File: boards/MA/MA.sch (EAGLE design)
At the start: 14 parts

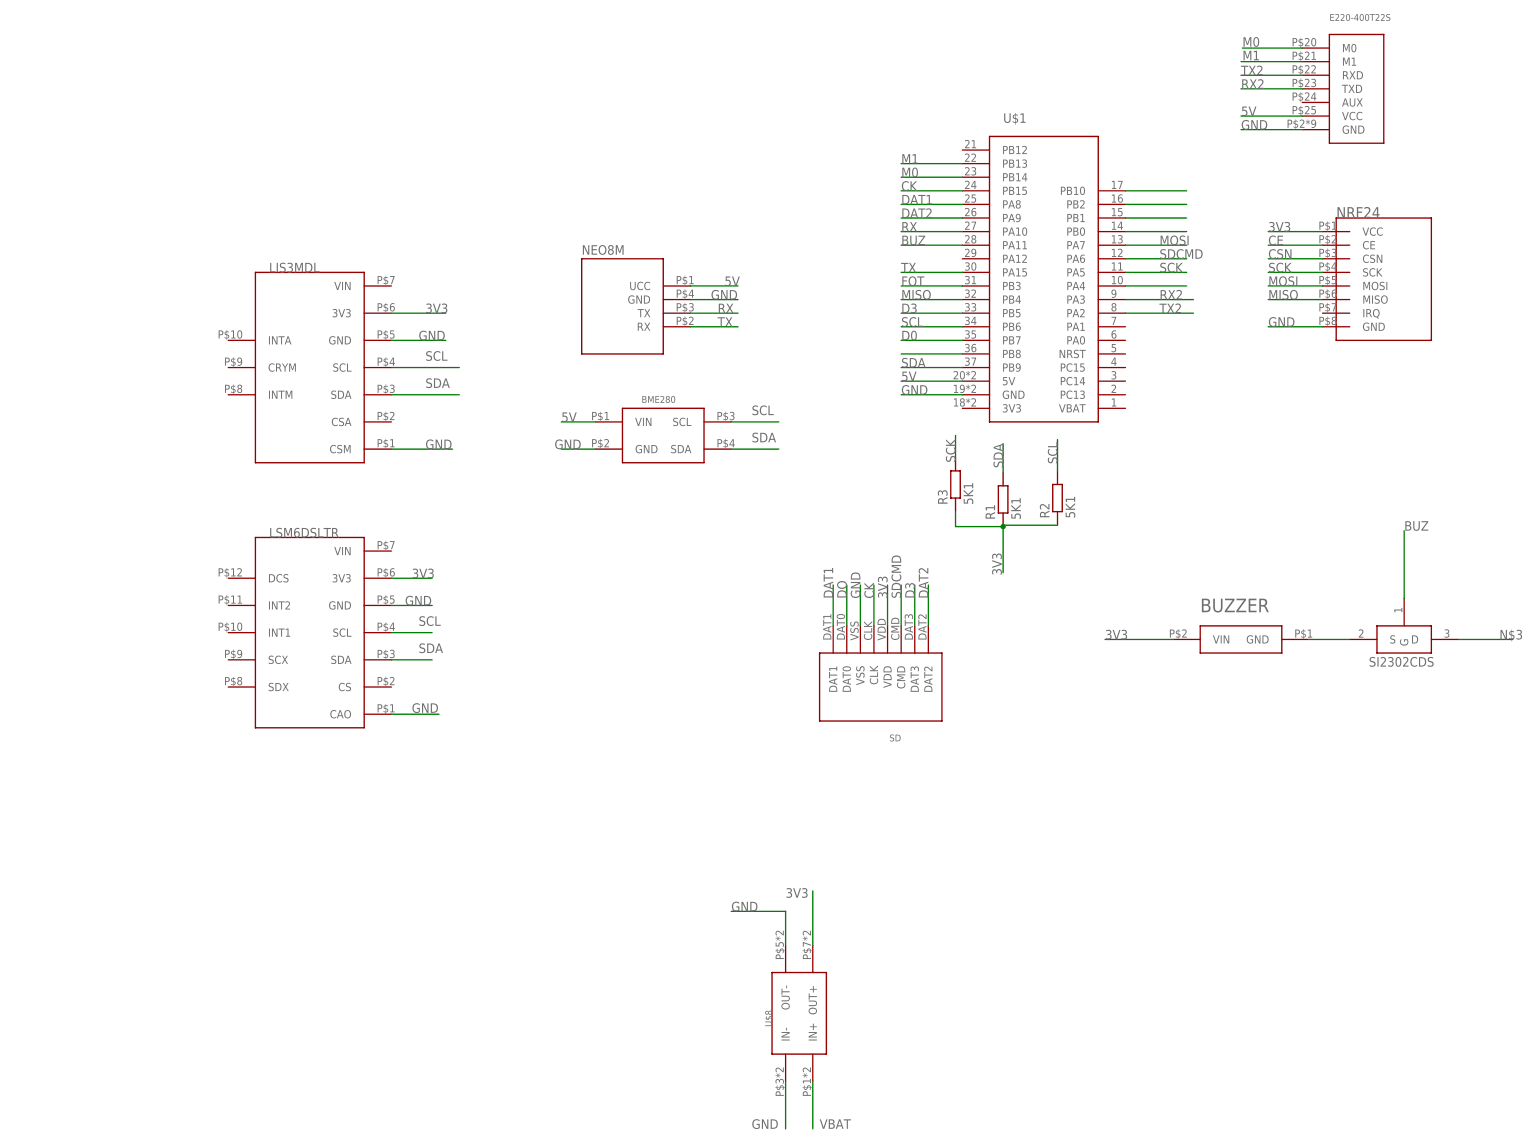
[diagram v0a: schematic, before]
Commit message: доделал платы до приемлемого уровня.
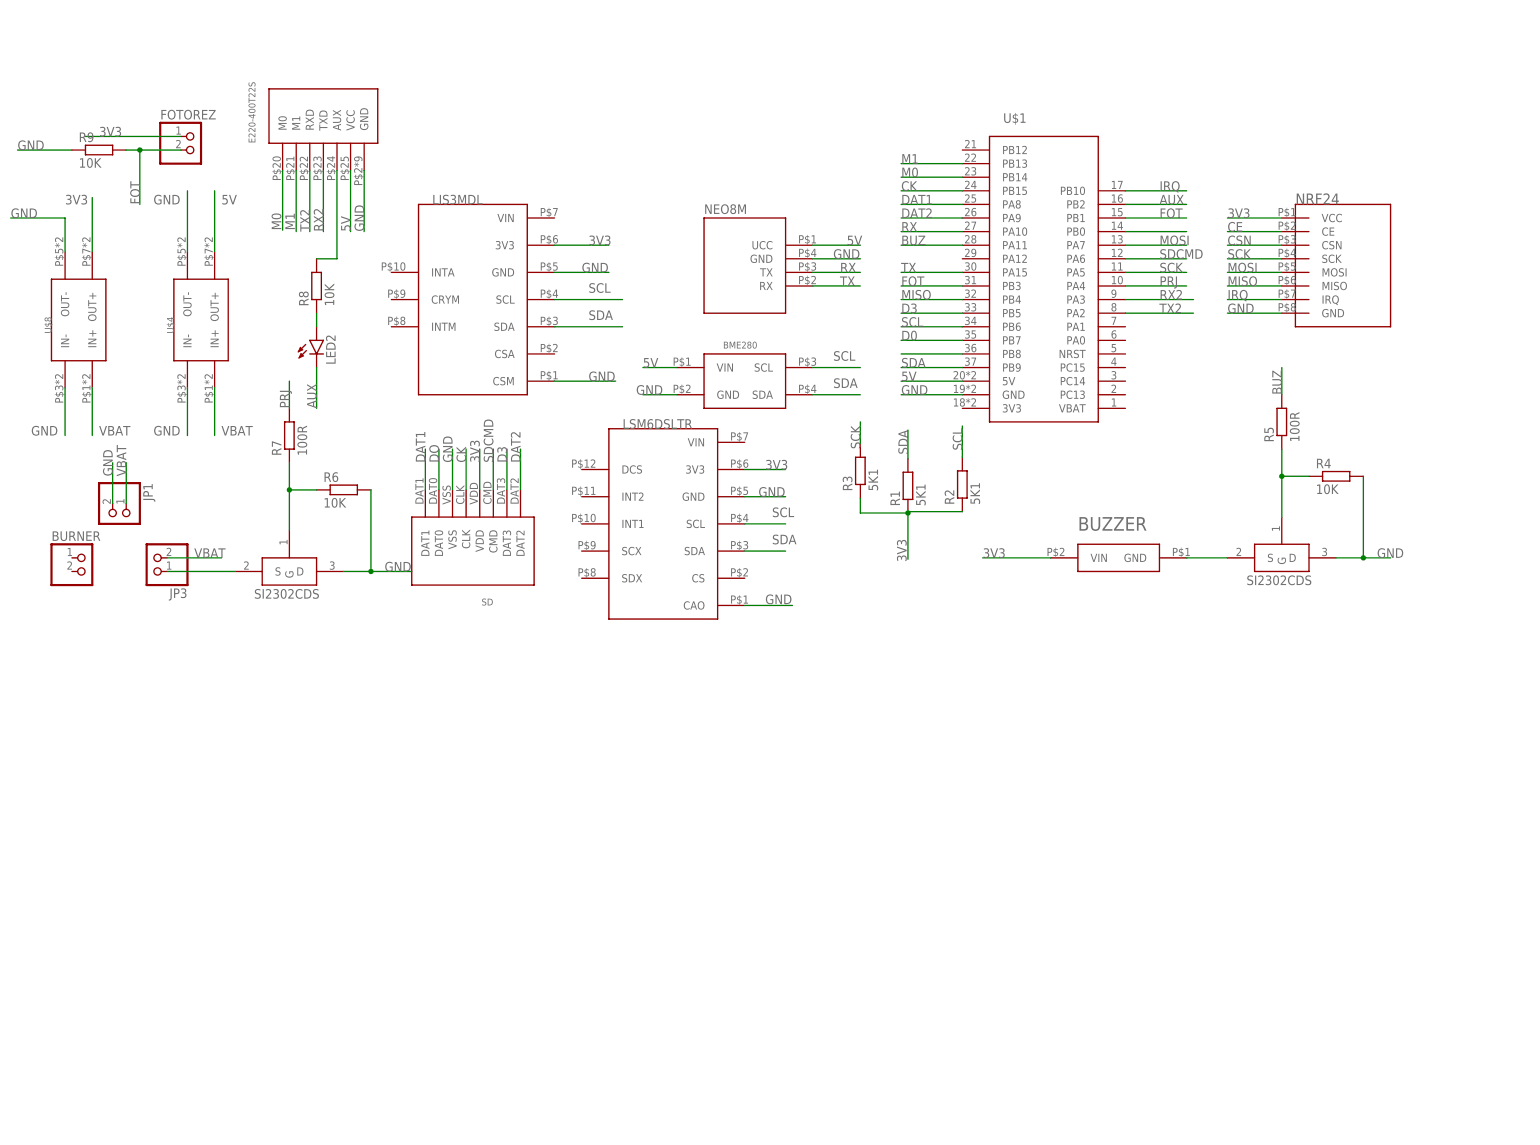
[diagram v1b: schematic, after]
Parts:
- added BURNER, FOTOREZ, JP1, JP3: (no value), pinhead:PINHD-1X2
- added LED2: (no value), led:LEDCHIP-LED0603
- added R4, R6, R8, R9: 10K, rcl:R-EU_R0603
- added R5, R7: 100R, rcl:R-EU_R0603
- added U$3: SI2302CDS, CanCubeSat:SI2302CDS
- added U$4: MP1584-B, UNKNOWN-2024:MP1584-B
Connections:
- removed net N$1: U$1.PB10
- removed net N$5: U$1.PB0
- removed net N$6: U$1.PB1
- removed net N$7: U$1.PB2
- removed net N$8: U$1.PA4
- new net AUX: LED2.C, U$1.PB2
- new net IRQ: NRF24.IRQ, U$1.PB10
- new net N$4: E220-400T22S.AUX, R8.2
- new net N$9: LED2.A, R8.1
- new net PRJ: R7.2, U$1.PA4
- net 3V3: now also FOTOREZ.1
- net 5V: now also U$4.OUT+
- net BUZ: now also R4.1, R5.1, R5.2, R6.1, R7.1, U$3.G
- net FOT: now also FOTOREZ.2, R9.2, U$1.PB0, U$1.PB1
- net GND: now also JP1.2, R4.2, R6.2, R9.1, U$2.D, U$3.D, U$4.IN-, U$4.OUT-
- net N$3: now also JP3.1, U$3.S; no longer U$2.D
- net VBAT: now also JP1.1, JP3.2, U$4.IN+
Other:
- moved on the sheet: BME280, BUZZER, E220-400T22S, LIS3MDL, LSM6DSLTR, NEO8M, NRF24, R1, R2, R3, SD, U$8
